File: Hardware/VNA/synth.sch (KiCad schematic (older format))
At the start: 32 parts, among them U3 MAX2871, X1 ASTXR-12-19.200MHz

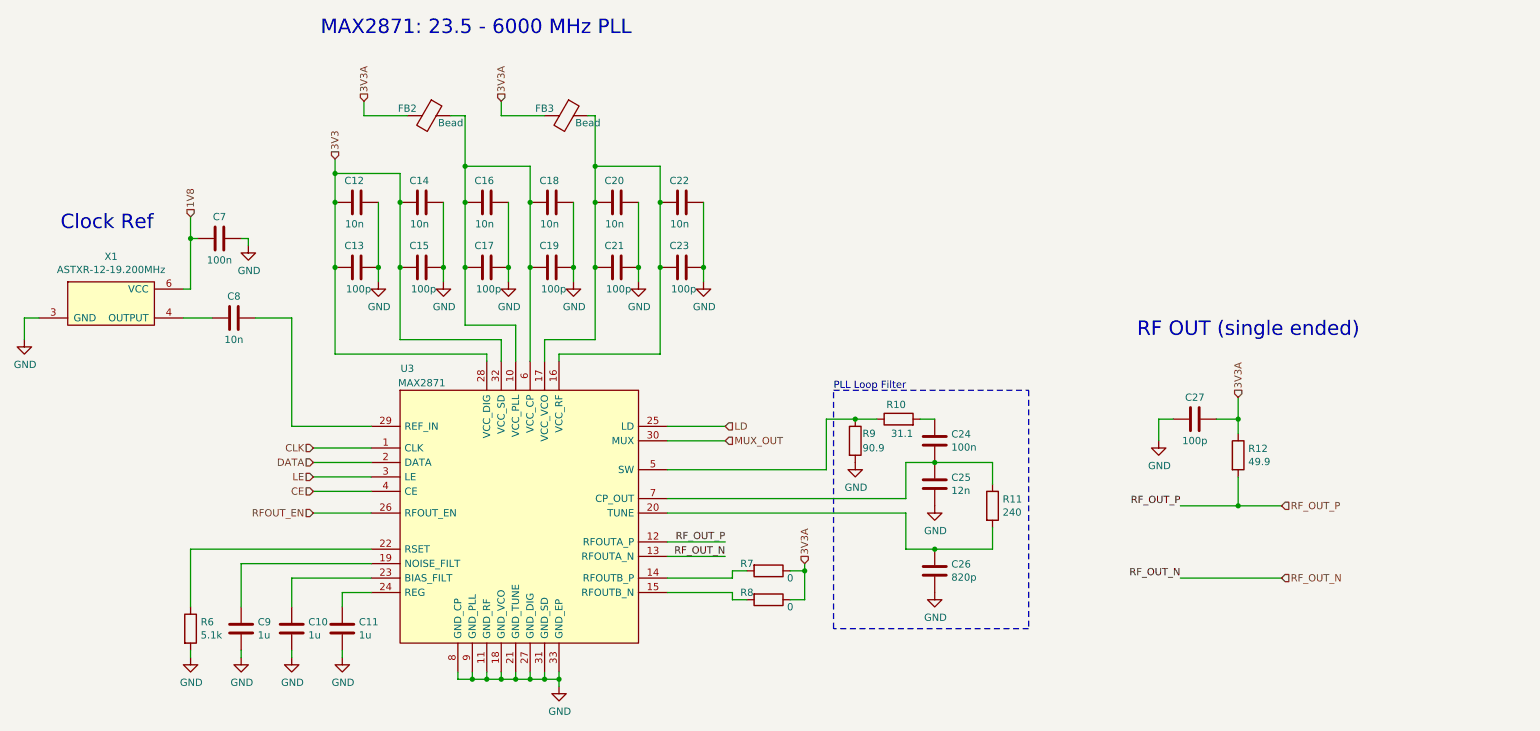
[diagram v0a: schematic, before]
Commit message: More schematic changes + updated functionals
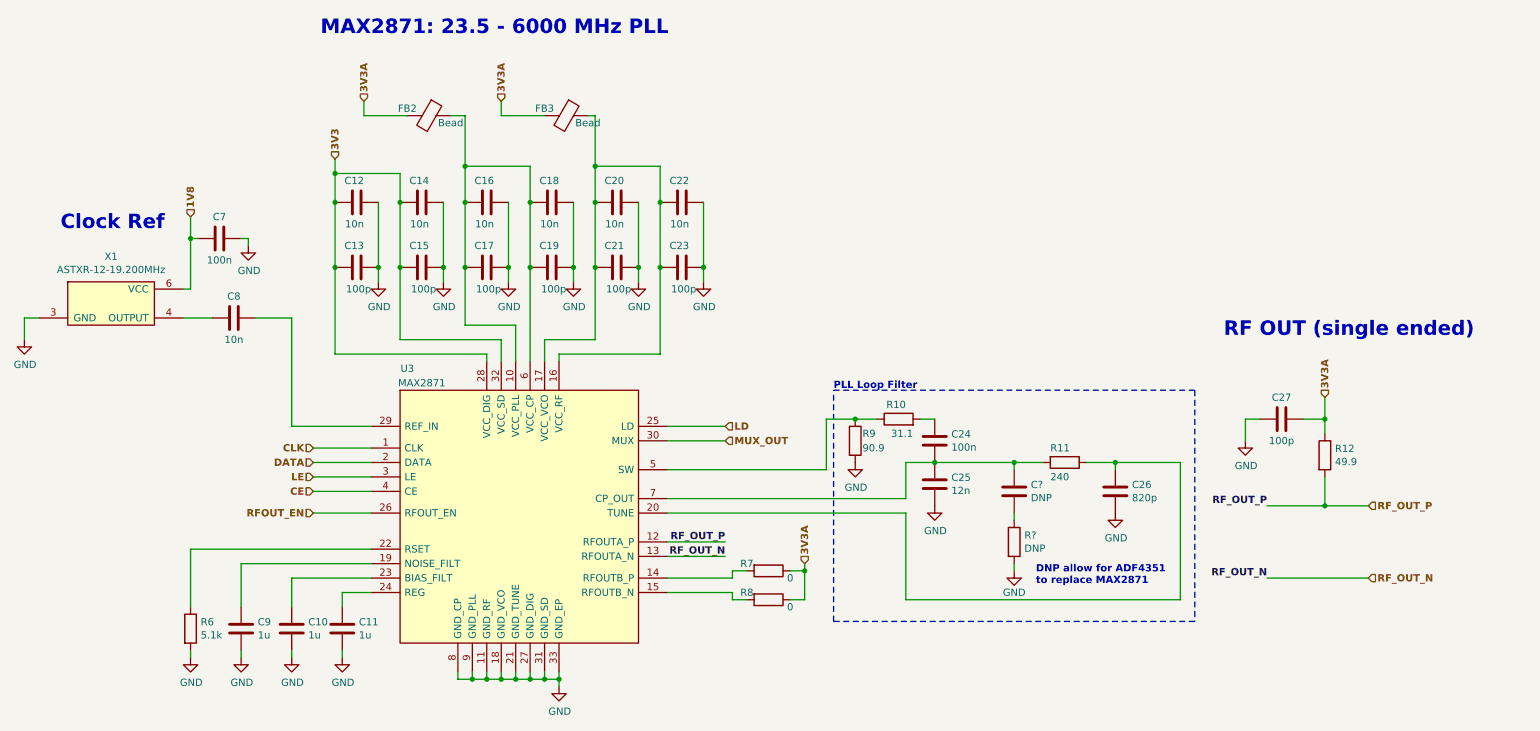
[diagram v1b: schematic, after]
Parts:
- added C?: DNP, symbol Device:C
- added R?: DNP, symbol Device:R
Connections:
- net GND: now also R?.2
- net at C26.1, U3.20 (TUNE): now also R11.1; no longer R11.2
- net at C24.2, C25.1, U3.7 (CP_OUT): now also R11.2, C?.1; no longer R11.1
- new net: C?.2, R?.1
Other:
- note added: "DNP allow for ADF4351\nto replace MAX2871"
- moved on the sheet: C26, C27, R11, R12
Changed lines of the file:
@@
 L Device:C C26
 U 1 1 5C44DD06
-P 7300 5050
-F 0 "C26" H 7415 5096 50  0000 L CNN
-F 1 "820p" H 7415 5005 50  0000 L CNN
-F 2 "Capacitor_SMD:C_0402_1005Metric" H 7338 4900 50  0001 C CNN
-F 3 "~" H 7300 5050 50  0001 C CNN
-	1    7300 5050
+P 8550 4500
+F 0 "C26" H 8665 4546 50  0000 L CNN
+F 1 "820p" H 8665 4455 50  0000 L CNN
+F 2 "Capacitor_SMD:C_0402_1005Metric" H 8588 4350 50  0001 C CNN
+F 3 "~" H 8550 4500 50  0001 C CNN
+	1    8550 4500
 	1    0    0    -1
 $EndComp
@@
 L power:GND #PWR027
 U 1 1 5C44DD0E
-P 7300 5200
-F 0 "#PWR027" H 7300 4950 50  0001 C CNN
-F 1 "GND" H 7305 5027 50  0000 C CNN
-F 2 "" H 7300 5200 50  0001 C CNN
-F 3 "" H 7300 5200 50  0001 C CNN
-	1    7300 5200
+P 8550 4650
+F 0 "#PWR027" H 8550 4400 50  0001 C CNN
+F 1 "GND" H 8555 4477 50  0000 C CNN
+F 2 "" H 8550 4650 50  0001 C CNN
+F 3 "" H 8550 4650 50  0001 C CNN
+	1    8550 4650
 	1    0    0    -1
 $EndComp
@@
 L Device:R R11
 U 1 1 5C45B711
-P 7700 4600
-F 0 "R11" H 7770 4646 50  0000 L CNN
-F 1 "240" H 7770 4555 50  0000 L CNN
-F 2 "Resistor_SMD:R_0402_1005Metric" V 7630 4600 50  0001 C CNN
-F 3 "~" H 7700 4600 50  0001 C CNN
-	1    7700 4600
-	1    0    0    -1
-$EndComp
-Wire Wire Line
-	7700 4300 7700 4450
+P 8200 4300
+F 0 "R11" V 8100 4200 50  0000 L CNN
+F 1 "240" V 8300 4200 50  0000 L CNN
+F 2 "Resistor_SMD:R_0402_1005Metric" V 8130 4300 50  0001 C CNN
+F 3 "~" H 8200 4300 50  0001 C CNN
+	1    8200 4300
+	0    1    1    0
+$EndComp
 Wire Wire Line
 	7100 4550 7100 4300
-Wire Wire Line
-	7100 4900 7100 4650
-Wire Wire Line
-	7700 4900 7700 4750
 Wire Wire Line
 	6550 4000 6550 4350
 Wire Notes Line
-	6600 3800 7950 3800
-Wire Notes Line
-	7950 3800 7950 5450
-Wire Notes Line
-	7950 5450 6600 5450
-Wire Notes Line
-	6600 5450 6600 3800
-Text Notes 6600 3800 0    50   ~ 0
+	6600 5400 6600 3800
+Text Notes 6600 3800 0    50   ~ 6
 PLL Loop Filter\n
 Wire Wire Line
@@
 Wire Wire Line
 	5450 4950 5850 4950
-Text Label 5850 4950 2    50   ~ 0
+Text Label 5850 4950 2    50   ~ 6
 RF_OUT_N
-Text Label 5850 4850 2    50   ~ 0
+Text Label 5850 4850 2    50   ~ 6
 RF_OUT_P
 Wire Wire Line
@@
 	4950 1900 4950 2250
 Connection ~ 4950 2250
-Text Label 9000 5100 2    50   ~ 0
+Text Label 9600 5100 2    50   ~ 6
 RF_OUT_N
-Text Label 9000 4600 2    50   ~ 0
+Text Label 9600 4600 2    50   ~ 6
 RF_OUT_P
 Wire Wire Line
@@
 L Device:R R12
 U 1 1 5C664064
-P 9400 4250
-F 0 "R12" H 9470 4296 50  0000 L CNN
-F 1 "49.9" H 9470 4205 50  0000 L CNN
-F 2 "Resistor_SMD:R_0402_1005Metric" V 9330 4250 50  0001 C CNN
-F 3 "~" H 9400 4250 50  0001 C CNN
-	1    9400 4250
+P 10000 4250
+F 0 "R12" H 10070 4296 50  0000 L CNN
+F 1 "49.9" H 10070 4205 50  0000 L CNN
+F 2 "Resistor_SMD:R_0402_1005Metric" V 9930 4250 50  0001 C CNN
+F 3 "~" H 10000 4250 50  0001 C CNN
+	1    10000 4250
 	1    0    0    -1
 $EndComp
@@
 L Device:C C27
 U 1 1 5C674D87
-P 9100 4000
-F 0 "C27" V 8950 4000 50  0000 C CNN
-F 1 "100p" V 9250 4000 50  0000 C CNN
-F 2 "Capacitor_SMD:C_0402_1005Metric" H 9138 3850 50  0001 C CNN
-F 3 "~" H 9100 4000 50  0001 C CNN
-	1    9100 4000
-	0    1    1    0
-$EndComp
-Wire Wire Line
-	9250 4000 9400 4000
-Wire Wire Line
-	8950 4000 8850 4000
-Wire Wire Line
-	8850 4000 8850 4150
+P 9700 4000
+F 0 "C27" V 9550 4000 50  0000 C CNN
+F 1 "100p" V 9850 4000 50  0000 C CNN
+F 2 "Capacitor_SMD:C_0402_1005Metric" H 9738 3850 50  0001 C CNN
+F 3 "~" H 9700 4000 50  0001 C CNN
+	1    9700 4000
+	0    1    1    0
+$EndComp
+Wire Wire Line
+	9850 4000 10000 4000
+Wire Wire Line
+	9550 4000 9450 4000
+Wire Wire Line
+	9450 4000 9450 4150
 $Comp
 L power:GND #PWR028
 U 1 1 5C6A88A2
-P 8850 4150
-F 0 "#PWR028" H 8850 3900 50  0001 C CNN
-F 1 "GND" H 8855 3977 50  0000 C CNN
-F 2 "" H 8850 4150 50  0001 C CNN
-F 3 "" H 8850 4150 50  0001 C CNN
-	1    8850 4150
-	1    0    0    -1
-$EndComp
-Connection ~ 9400 4000
-Wire Wire Line
-	9400 4000 9400 4100
-Wire Wire Line
-	9400 3850 9400 4000
+P 9450 4150
+F 0 "#PWR028" H 9450 3900 50  0001 C CNN
+F 1 "GND" H 9455 3977 50  0000 C CNN
+F 2 "" H 9450 4150 50  0001 C CNN
+F 3 "" H 9450 4150 50  0001 C CNN
+	1    9450 4150
+	1    0    0    -1
+$EndComp
+Connection ~ 10000 4000
+Wire Wire Line
+	10000 4000 10000 4100
+Wire Wire Line
+	10000 3850 10000 4000
 Wire Wire Line
 	3350 1900 3350 1800
@@
 Wire Wire Line
 	5450 5100 5900 5100
-Text Notes 8700 3600 0    100  ~ 0
+Text Notes 9300 3600 0    100  ~ 6
 RF OUT (single ended)\n\n
 Wire Wire Line
@@
 	1    0    0    -1
 $EndComp
-Text Notes 1250 2700 0    100  ~ 0
+Text Notes 1250 2700 0    100  ~ 6
 Clock Ref\n
 Wire Wire Line
@@
 $EndComp
 Wire Wire Line
-	9000 4600 9400 4600
+	9600 4600 10000 4600
 $Comp
 L VNA_Symbols:ASTXR-12-19.200MHz X1
@@
 $EndComp
 Wire Wire Line
-	9000 5100 9700 5100
-Wire Wire Line
-	9400 4400 9400 4600
-Connection ~ 9400 4600
-Wire Wire Line
-	9400 4600 9700 4600
+	9600 5100 10300 5100
+Wire Wire Line
+	10000 4400 10000 4600
+Connection ~ 10000 4600
+Wire Wire Line
+	10000 4600 10300 4600
 Wire Wire Line
 	3900 2500 3900 2950
@@
 	7100 4300 7300 4300
 Wire Wire Line
-	7100 4900 7300 4900
-Wire Wire Line
 	6550 4000 6750 4000
 Wire Wire Line
@@
 Wire Wire Line
 	3150 2300 3150 2500
-Text HLabel 9700 4600 2    50   Input ~ 0
+Text HLabel 10300 4600 2    50   Input ~ 6
 RF_OUT_P
-Text HLabel 9700 5100 2    50   Input ~ 0
+Text HLabel 10300 5100 2    50   Input ~ 6
 RF_OUT_N
-Text HLabel 5850 4050 2    50   Input ~ 0
+Text HLabel 5850 4050 2    50   Input ~ 6
 LD
-Text HLabel 5850 4150 2    50   Input ~ 0
+Text HLabel 5850 4150 2    50   Input ~ 6
 MUX_OUT
-Text HLabel 3000 4200 0    50   Input ~ 0
+Text HLabel 3000 4200 0    50   Input ~ 6
 CLK
-Text HLabel 3000 4300 0    50   Input ~ 0
+Text HLabel 3000 4300 0    50   Input ~ 6
 DATA
-Text HLabel 3000 4400 0    50   Input ~ 0
+Text HLabel 3000 4400 0    50   Input ~ 6
 LE
-Text HLabel 3000 4500 0    50   Input ~ 0
+Text HLabel 3000 4500 0    50   Input ~ 6
 CE
-Text HLabel 3000 4650 0    50   Input ~ 0
+Text HLabel 3000 4650 0    50   Input ~ 6
 RFOUT_EN
 Connection ~ 3150 2500
@@
 	6750 4000 6900 4000
 Connection ~ 7300 4300
-Wire Wire Line
-	7300 4300 7700 4300
-Connection ~ 7300 4900
-Wire Wire Line
-	7300 4900 7700 4900
-Text Notes 3050 1350 0    100  ~ 0
+Text Notes 3050 1350 0    100  ~ 6
 MAX2871: 23.5 - 6000 MHz PLL\n
-Text HLabel 9400 3850 1    50   Input ~ 0
+Text HLabel 10000 3850 1    50   Input ~ 6
 3V3A
-Text HLabel 2150 2600 1    50   Input ~ 0
+Text HLabel 2150 2600 1    50   Input ~ 6
 1V8
-Text HLabel 3350 1800 1    50   Input ~ 0
+Text HLabel 3350 1800 1    50   Input ~ 6
 3V3A
-Text HLabel 4300 1800 1    50   Input ~ 0
+Text HLabel 4300 1800 1    50   Input ~ 6
 3V3A
-Text HLabel 6400 5000 1    50   Input ~ 0
+Text HLabel 6400 5000 1    50   Input ~ 6
 3V3A
-Text HLabel 3150 2200 1    50   Input ~ 0
+Text HLabel 3150 2200 1    50   Input ~ 6
 3V3
 $Comp
@@
 	0    1    1    0
 $EndComp
+Wire Wire Line
+	7300 4300 7850 4300
+$Comp
+L Device:C C?
+U 1 1 5CB618D9
+P 7850 4500
+F 0 "C?" H 7965 4546 50  0000 L CNN
+F 1 "DNP" H 7965 4455 50  0000 L CNN
+F 2 "" H 7888 4350 50  0001 C CNN
+F 3 "~" H 7850 4500 50  0001 C CNN
+	1    7850 4500
+	1    0    0    -1
+$EndComp
+$Comp
+L Device:R R?
+U 1 1 5CB620B8
+P 7850 4850
+F 0 "R?" H 7920 4896 50  0000 L CNN
+F 1 "DNP" H 7920 4805 50  0000 L CNN
+F 2 "" V 7780 4850 50  0001 C CNN
+F 3 "~" H 7850 4850 50  0001 C CNN
+	1    7850 4850
+	1    0    0    -1
+$EndComp
+Wire Wire Line
+	8550 4300 8550 4350
+Connection ~ 8550 4300
+Wire Wire Line
+	8550 4300 8350 4300
+Wire Wire Line
+	7850 4300 7850 4350
+Connection ~ 7850 4300
+Wire Wire Line
+	7850 4300 8050 4300
+Wire Wire Line
+	7850 4650 7850 4700
+Wire Wire Line
+	7850 5000 7850 5050
+Wire Wire Line
+	9000 4300 9000 5250
+Wire Wire Line
+	9000 5250 7100 5250
+Wire Wire Line
+	7100 4650 7100 5250
+Wire Wire Line
+	8550 4300 9000 4300
+$Comp
+L power:GND #PWR?
+U 1 1 5CB860A2
+P 7850 5050
+F 0 "#PWR?" H 7850 4800 50  0001 C CNN
+F 1 "GND" H 7850 4900 50  0000 C CNN
+F 2 "" H 7850 5050 50  0001 C CNN
+F 3 "" H 7850 5050 50  0001 C CNN
+	1    7850 5050
+	1    0    0    -1
+$EndComp
+Wire Notes Line
+	6600 3800 9100 3800
+Wire Notes Line
+	9100 3800 9100 5400
+Wire Notes Line
+	9100 5400 6600 5400
+Text Notes 8000 5150 0    50   ~ 6
+DNP allow for ADF4351\nto replace MAX2871
 $EndSCHEMATC
